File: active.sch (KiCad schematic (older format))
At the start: 33 parts, among them P1 CONN_1, P10 CONN_1, P11 CONN_1, P12 CONN_1, P2 CONN_1, P3 CONN_1, P4 CONN_1, P5 CONN_1, P6 CONN_1, P7 CONN_1, P8 SPI, P9 CONN_4, U1 ADS1291/2

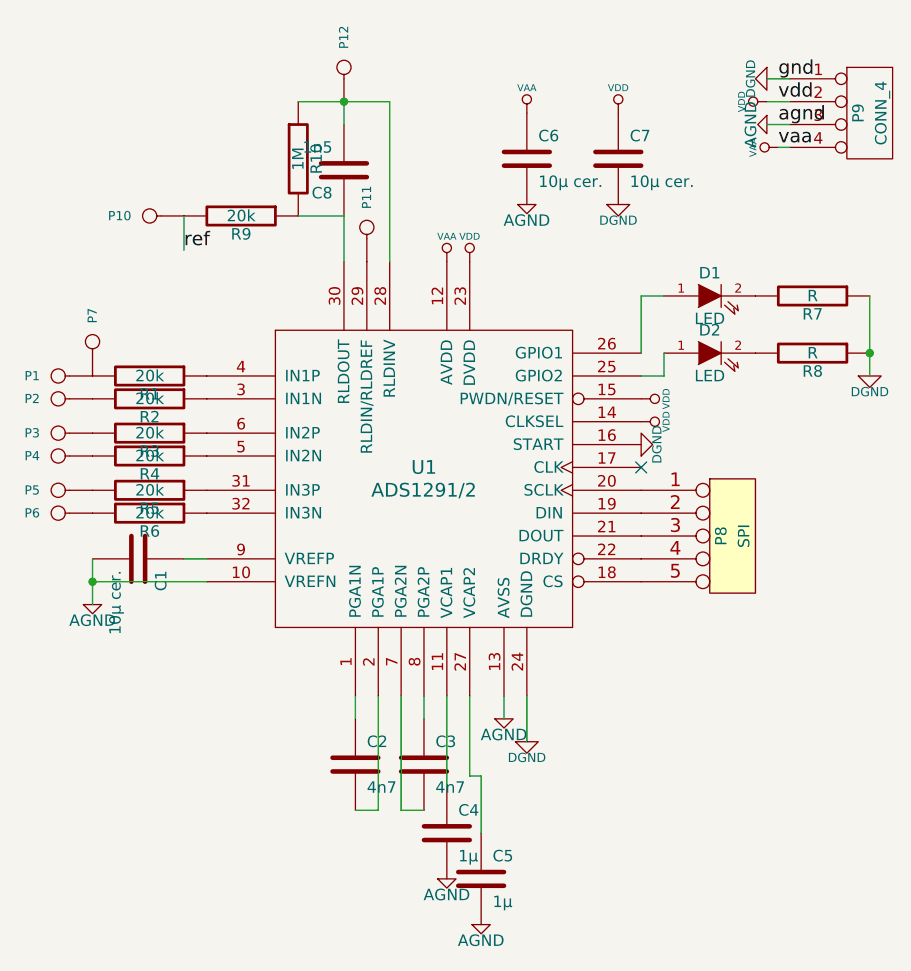
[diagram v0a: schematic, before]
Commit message: small clarification in the schmematic
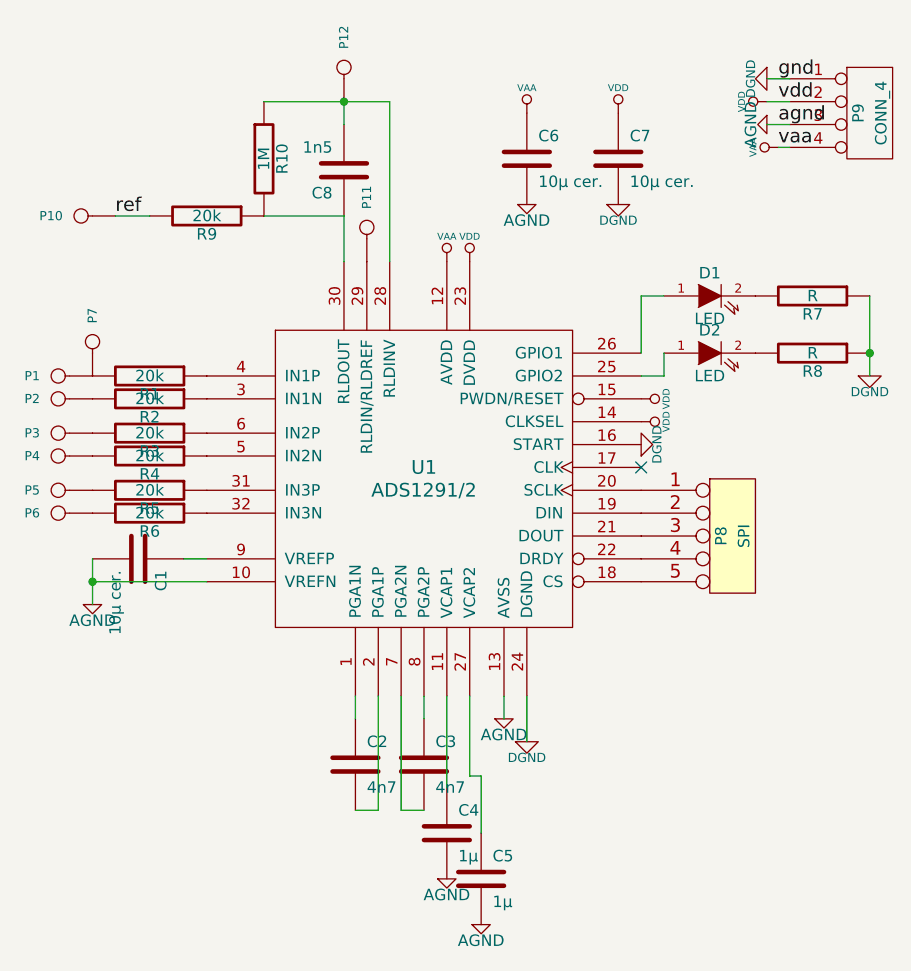
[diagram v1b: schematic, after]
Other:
- moved on the sheet: P10, R10, R9
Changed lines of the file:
@@
-EESchema Schematic File Version 2  date Thu 16 Feb 2012 12:05:28 PM CET
+EESchema Schematic File Version 2  date Thu 16 Feb 2012 12:25:49 PM CET
 LIBS:power
 LIBS:device
@@
 	5000 2600 5000 1900
 Wire Wire Line
-	5000 1900 4600 1900
+	5000 1900 4800 1900
 Wire Wire Line
-	4600 2400 4800 2400
+	4800 1900 4450 1900
+Wire Wire Line
+	4450 2400 4800 2400
 Wire Wire Line
 	6750 2100 6700 2100
@@
 Connection ~ 7100 3000
 Wire Wire Line
-	7100 2750 7100 3100
+	7100 2750 7100 3000
+Wire Wire Line
+	7100 3000 7100 3100
 Connection ~ 3700 4000
 Wire Wire Line
-	3700 3900 3700 4100
+	3700 3900 3700 4000
+Wire Wire Line
+	3700 4000 3700 4100
 Wire Wire Line
 	5400 5100 5400 4850
@@
 	4800 1900 4800 2000
 Wire Wire Line
-	4100 2400 4100 2550
+	3950 2400 3800 2400
 Wire Wire Line
 	6650 1900 6750 1900
-Text Label 4100 2550 0    60   ~ 0
+Text Label 3800 2400 0    60   ~ 0
 ref
 $Comp
@@
 L CONN_1 P10
 U 1 1 4EFD05E7
-P 3950 2400
-F 0 "P10" H 4030 2400 40  0000 L CNN
-F 1 "CONN_1" H 3950 2455 30  0001 C CNN
-	1    3950 2400
+P 3650 2400
+F 0 "P10" H 3730 2400 40  0000 L CNN
+F 1 "CONN_1" H 3650 2455 30  0001 C CNN
+	1    3650 2400
 	-1   0    0    1
 $EndComp
@@
 L R R9
 U 1 1 4EFD05B9
-P 4350 2400
-F 0 "R9" V 4430 2400 50  0000 C CNN
-F 1 "20k" V 4350 2400 50  0000 C CNN
-	1    4350 2400
+P 4200 2400
+F 0 "R9" V 4280 2400 50  0000 C CNN
+F 1 "20k" V 4200 2400 50  0000 C CNN
+	1    4200 2400
 	0    1    1    0
 $EndComp
@@
 L R R10
 U 1 1 4EFD043C
-P 4600 2150
-F 0 "R10" V 4680 2150 50  0000 C CNN
-F 1 "1M" V 4600 2150 50  0000 C CNN
-	1    4600 2150
+P 4450 2150
+F 0 "R10" V 4530 2150 50  0000 C CNN
+F 1 "1M" V 4450 2150 50  0000 C CNN
+	1    4450 2150
 	1    0    0    -1
 $EndComp
